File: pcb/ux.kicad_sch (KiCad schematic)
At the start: 53 parts, among them J7 GameBoy_LinkPort, J8 Conn_01x02, J9 Conn_01x40_MountingPin, SW1 AGB_DPAD, SW2 BOOT, SW3 RESET, SW4 AGB_AB, SW5 AGB_SELECT_START, U10 PI4IOE5V6416, U5 AP2502, U7 ICM-42670-P, U9 MAX98357

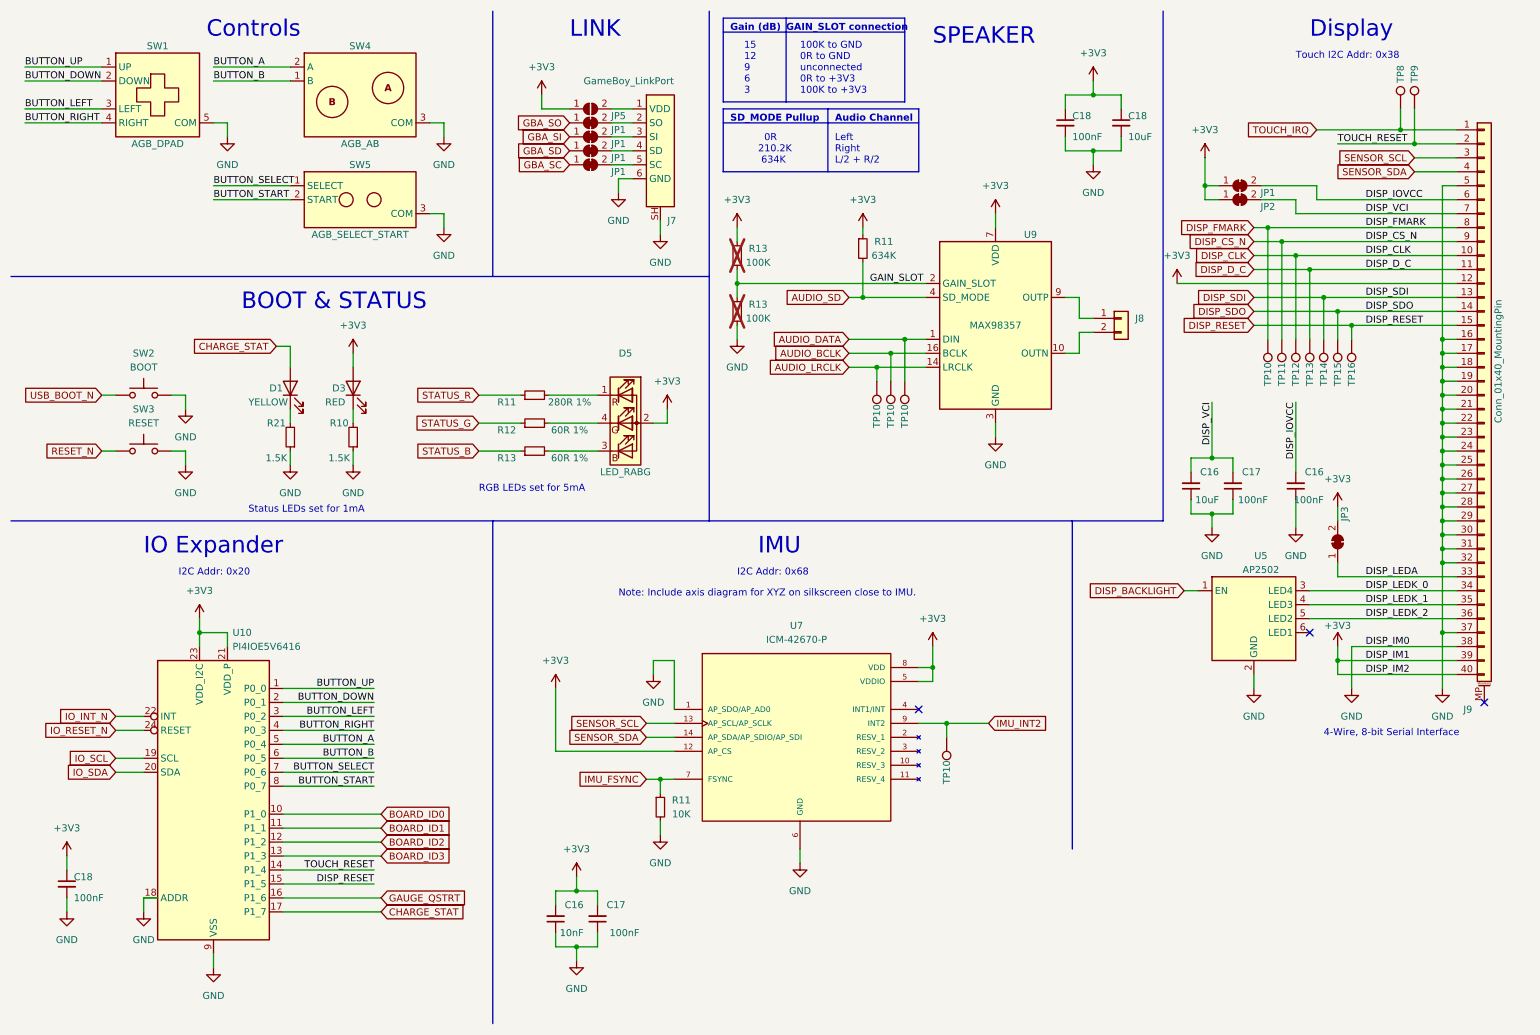
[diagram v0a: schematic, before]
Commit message: pcb: rev 0-r1 - board routed
Change-Id: Icb9c0ddbcf21cc7f2bac7bbcd371ff5a97baf35d
Reviewed-on: https://pigweed-review.googlesource.com/c/pigweed/kudzu/+/170233
Reviewed-by: Anthony DiGirolamo <tonymd@google.com>
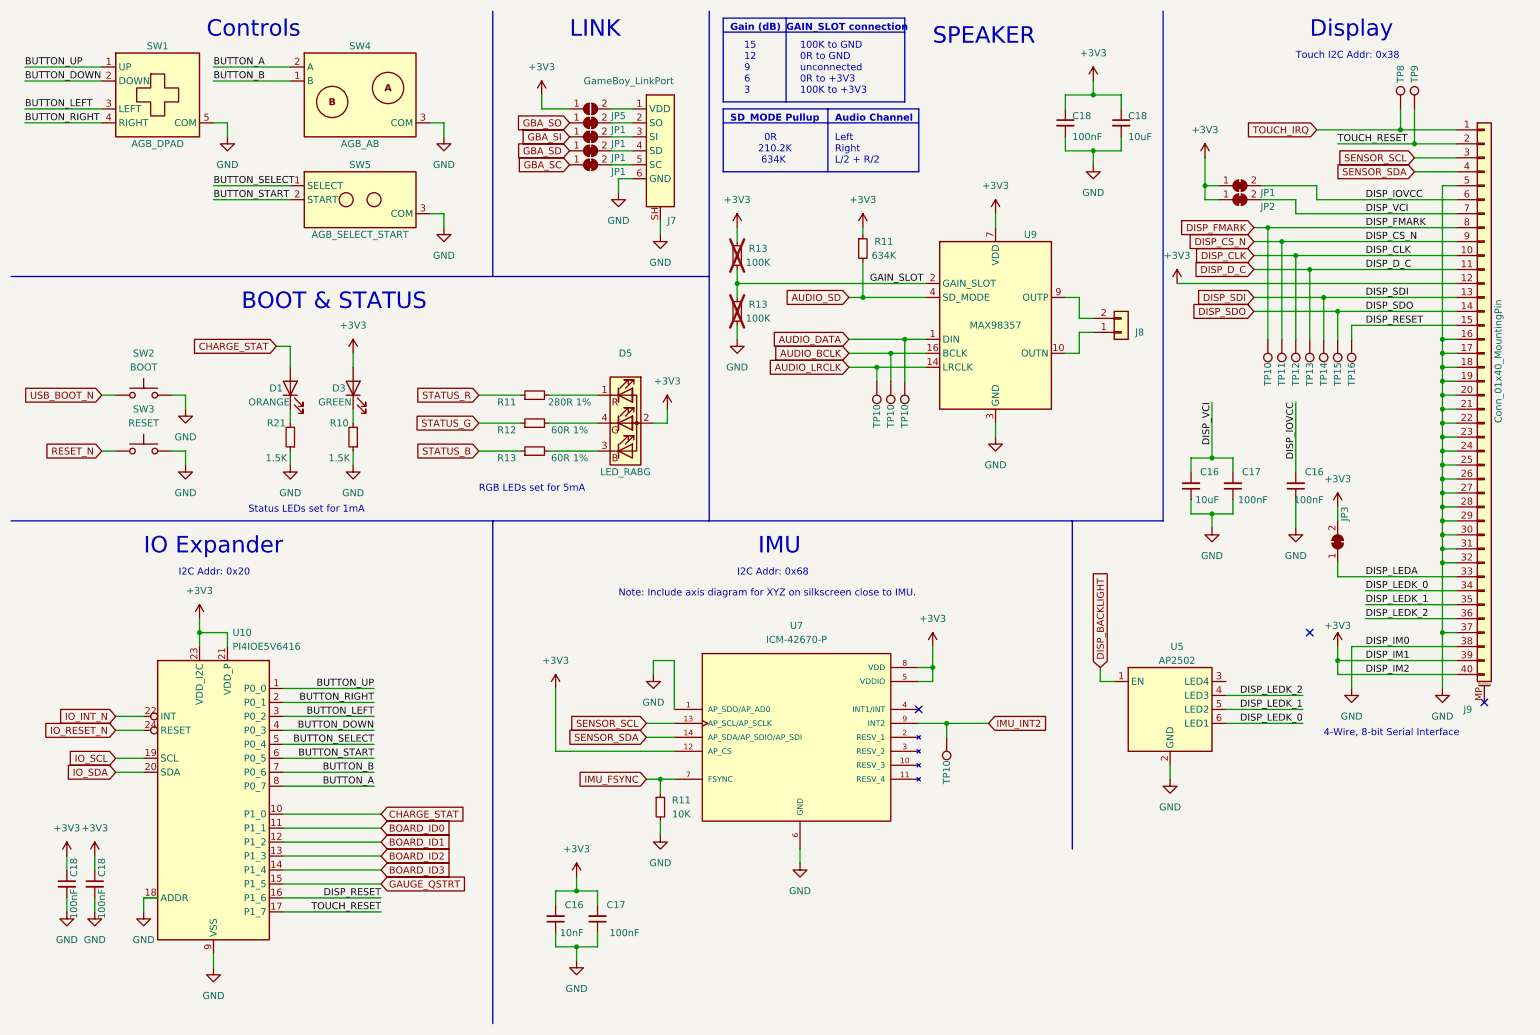
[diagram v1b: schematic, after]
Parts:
- added C18: 100nF, Capacitor_SMD:C_0603_1608Metric, symbol Device:C_Small
- D1: value YELLOW -> ORANGE; DigiKey PN (none) -> 160-1477-1-ND; Price @ 10 (none) -> 0.12700; Price @ 25 (none) -> 0.12700
- D3: value RED -> GREEN; DigiKey PN (none) -> 160-1475-1-ND; Price @ 10 (none) -> 0.13200; Price @ 25 (none) -> 0.13200
- D5: DigiKey PN 1830-1116-1-ND -> CLVBA-FKA-CA1D181BB7R3R3DKR-ND; Price @ 10 0.30300 -> 0.60000; Price @ 25 0.17420 -> 0.60000
- J8: footprint Connector_Molex:Molex_PicoBlade_53048-0210_1x02_P1.25mm_Horizontal -> KudzuLibrary:CONN HEADER SMD 2POS 1.25MM; DigiKey PN (none) -> WM7620CT-ND; Price @ 10 (none) -> 0.48300; Price @ 25 (none) -> 0.48300
- SW2, SW3: footprint Button_Switch_SMD:SW_Push_1P1T_NO_CK_KMR2 -> KudzuLibrary:SW_Push_1P1T_NO_CK_PTS840_GK_SMTR_LFS; DigiKey PN 401-1427-1-ND -> CKN10508CT-ND; Price @ 10 0.50700 -> 0.43900; Price @ 25 0.48840 -> 0.41360
- U10: footprint Package_DFN_QFN:TQFN-24-1EP_4x4mm_P0.5mm_EP2.1x2.1mm_ThermalVias -> Package_DFN_QFN:TQFN-24-1EP_4x4mm_P0.5mm_EP2.1x2.1mm
- U9: footprint Package_DFN_QFN:TQFN-16-1EP_3x3mm_P0.5mm_EP1.23x1.23mm_ThermalVias -> Package_DFN_QFN:TQFN-16-1EP_3x3mm_P0.5mm_EP1.23x1.23mm
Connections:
- net +3V3: now also C18.1
- net BOARD_ID0: now also U10.11 (P1_1); no longer U10.10 (P1_0)
- net BOARD_ID1: now also U10.12 (P1_2); no longer U10.11 (P1_1)
- net BOARD_ID2: now also U10.13 (P1_3); no longer U10.12 (P1_2)
- net BOARD_ID3: now also U10.14 (P1_4); no longer U10.13 (P1_3)
- net BUTTON_A: now also U10.8 (P0_7); no longer U10.5 (P0_4)
- net BUTTON_B: now also U10.7 (P0_6); no longer U10.6 (P0_5)
- net BUTTON_DOWN: now also U10.4 (P0_3); no longer U10.2 (P0_1)
- net BUTTON_RIGHT: now also U10.2 (P0_1); no longer U10.4 (P0_3)
- net BUTTON_SELECT: now also U10.5 (P0_4); no longer U10.7 (P0_6)
- net BUTTON_START: now also U10.6 (P0_5); no longer U10.8 (P0_7)
- net CHARGE_STAT: now also U10.10 (P1_0); no longer U10.17 (P1_7)
- net DISP_LEDK_0: now also U5.6 (LED1); no longer U5.3 (LED4)
- net DISP_LEDK_1: now also U5.5 (LED2); no longer U5.4 (LED3)
- net DISP_LEDK_2: now also U5.4 (LED3); no longer U5.5 (LED2)
- net DISP_RESET: now also U10.16 (P1_6); no longer U10.15 (P1_5)
- net GAUGE_QSTRT: now also U10.15 (P1_5); no longer U10.16 (P1_6)
- net GND: now also C18.2
- net TOUCH_RESET: now also U10.17 (P1_7); no longer U10.14 (P1_4)
- net at J8.1 (Pin_1): now also U9.10 (OUTN); no longer U9.9 (OUTP)
- net at J8.2 (Pin_2): now also U9.9 (OUTP); no longer U9.10 (OUTN)
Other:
- company: (none) -> Copyright 2023 The Pigweed Authors
- moved on the sheet: U5
